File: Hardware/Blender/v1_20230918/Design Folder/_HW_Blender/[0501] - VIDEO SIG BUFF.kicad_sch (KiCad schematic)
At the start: 6 parts, among them U1201 MIC920YC5-TR

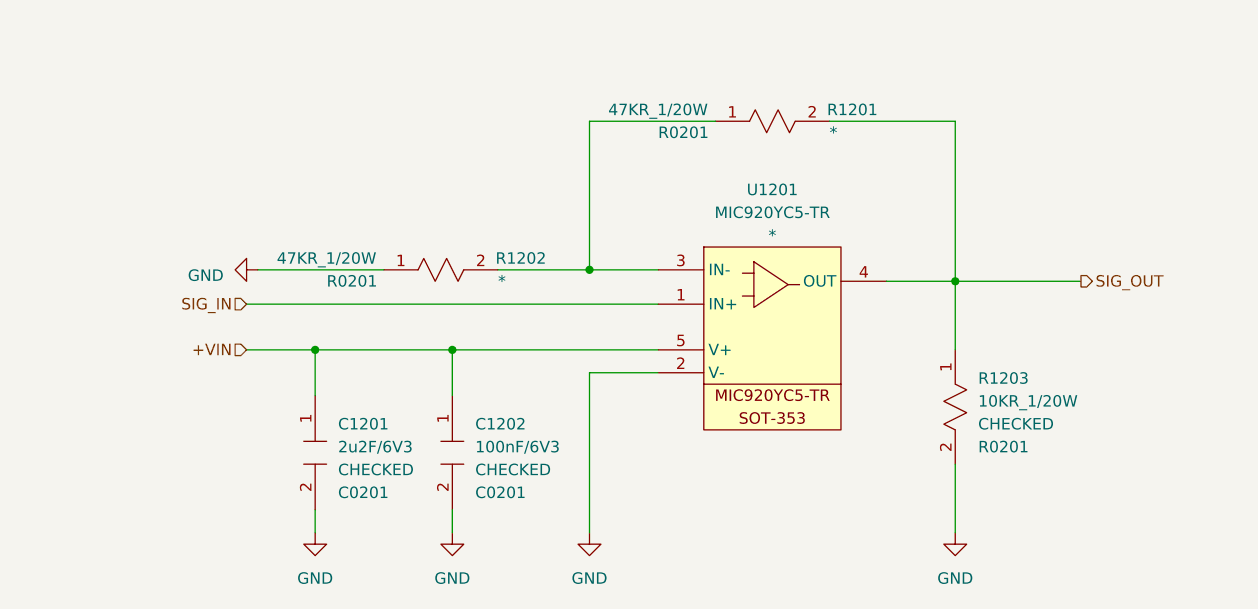
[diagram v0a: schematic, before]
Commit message: More update for hardware part
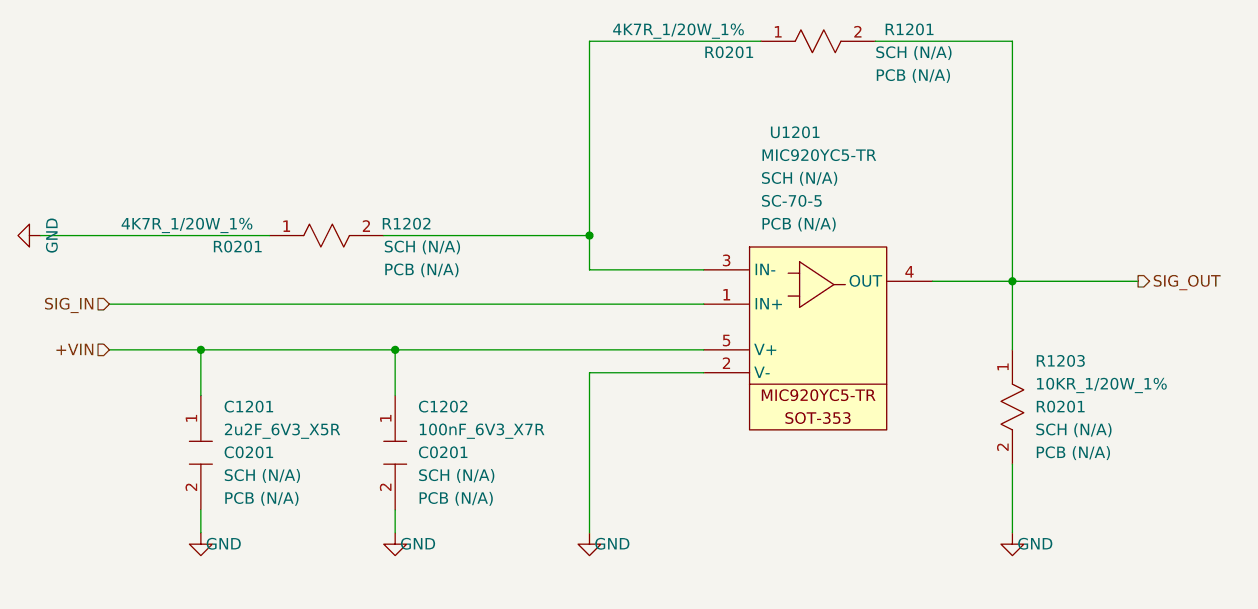
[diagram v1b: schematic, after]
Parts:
- C1201: value 2u2F/6V3 -> 2u2F_6V3_X5R; symbol _SCHLIB_Blender:CAP_2u2F/6V3_C0201 -> _SCHLIB_Blender:CAP_2u2F_6V3_X5R_C0201; Manufacturer (none) -> KYOCERA AVX; PCB CHECk (none) -> PCB (N/A); Part Number CM03X5R225M06AH -> (none); Part Number (Manufacturer) (none) -> CM03X5R225M06AH; Part Number (Vendor) (none) -> 478-KGM03CR50J225MHTR-ND; SCH CHECK CHECKED -> SCH (N/A); Vendor (none) -> Digikey
- C1202: value 100nF/6V3 -> 100nF_6V3_X7R; symbol _SCHLIB_Blender:CAP_100nF/6V3_C0201 -> _SCHLIB_Blender:CAP_100nF_6V3_X7R_C0201; Manufacturer (none) -> YAGEO; PCB CHECk (none) -> PCB (N/A); Part Number CC0201KRX7R5BB104 -> (none); Part Number (Manufacturer) (none) -> CC0201KRX7R5BB104; Part Number (Vendor) (none) -> 13-CC0201KRX7R5BB104TR-ND; SCH CHECK CHECKED -> SCH (N/A); Vendor (none) -> Digikey
- R1201, R1202: value 47KR_1/20W -> 4K7R_1/20W_1%; symbol _SCHLIB_Blender:RES_47KR_1/20W_R0201 -> _SCHLIB_Blender:RES_4K7R_1/20W_1%_R0201; Link https://www.digikey.ca/en/products/detail/yageo/AC0201FR-07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 -> https://www.digikey.ca/en/products/detail/stackpole-electro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; Manufacturer (none) -> Stackpole Electronics Inc; PCB CHECk (none) -> PCB (N/A); Part Number AC0201FR-0747KL -> (none); Part Number (Manufacturer) (none) -> RMCF0201FT4K70; Part Number (Vendor) (none) -> RMCF0201FT4K70TR-ND; SCH CHECK * -> SCH (N/A); Vendor (none) -> Digikey
- R1203: value 10KR_1/20W -> 10KR_1/20W_1%; symbol _SCHLIB_Blender:RES_10KR_1/20W-R0201 -> _SCHLIB_Blender:RES_10KR_1/20W_1%_R0201; Manufacturer (none) -> Stackpole Electronics Inc; PCB CHECk (none) -> PCB (N/A); Part Number RMCF0201FT10K0 -> (none); Part Number (Manufacturer) (none) -> RMCF0201FT10K0; Part Number (Vendor) (none) -> RMCF0201FT10K0TR-ND; SCH CHECK CHECKED -> SCH (N/A); Vendor (none) -> Digikey
- U1201: symbol _SCHLIB_ToslinkToDMX:OPAMP_MIC920YC5-TR -> _SCHLIB_Blender:IC_OPAMP_MIC920YC5-TR_GP_1C_5V~18V_SC-70-5; Manufacturer (none) -> Microchip Technology; PCB CHECk (none) -> PCB (N/A); Package (none) -> SC-70-5; Part Number MIC920YC5-TR -> (none); Part Number (Manufacturer) (none) -> MIC920YC5-TR; Part Number (Vendor) (none) -> 576-4560-2-ND; SCH CHECK * -> SCH (N/A); Vendor (none) -> Digikey
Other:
- moved on the sheet: C1201, C1202, R1201, R1202, R1203, U1201
